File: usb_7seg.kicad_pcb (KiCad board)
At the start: 2 copper layers, 72 x 47 mm, 8 parts, among them IC1 MAX7219CNG, IC2 MAX7219CWG, U1 SeeeduinoXIAO, U2 7segment_led

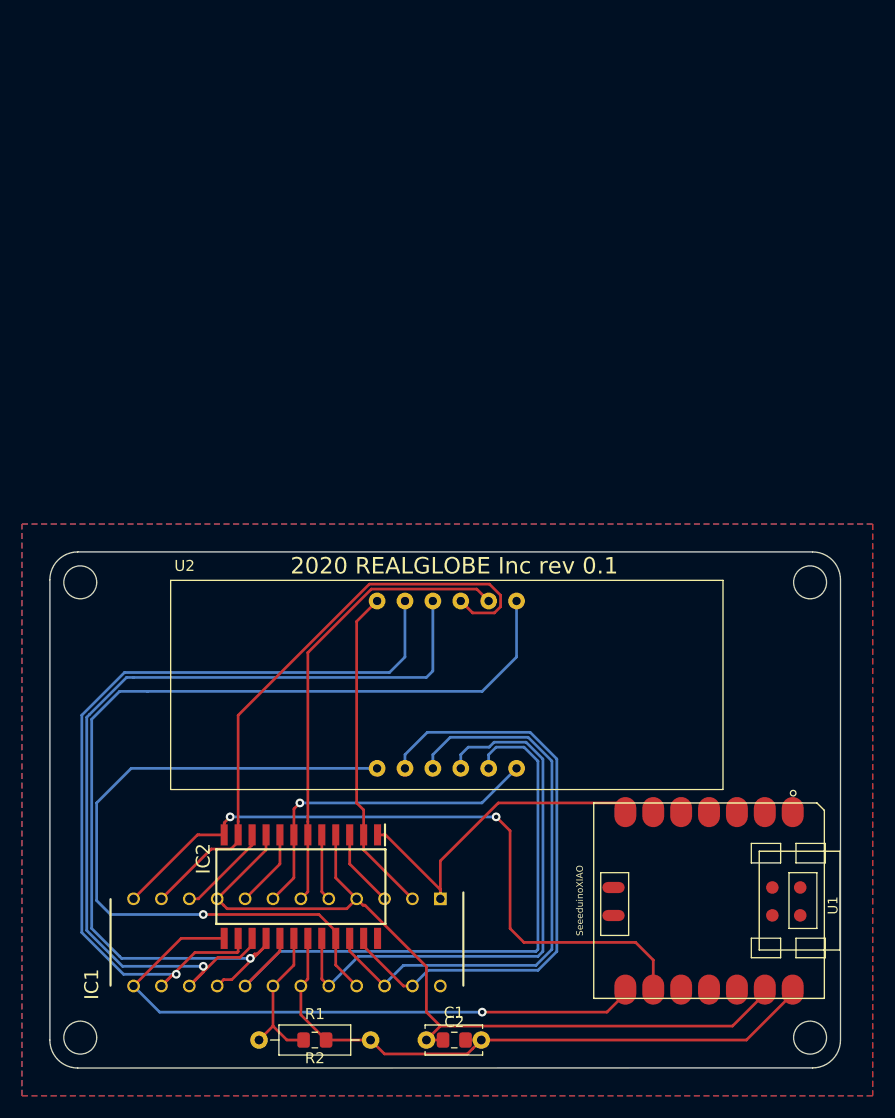
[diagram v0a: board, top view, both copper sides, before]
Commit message: いろいろ修正した
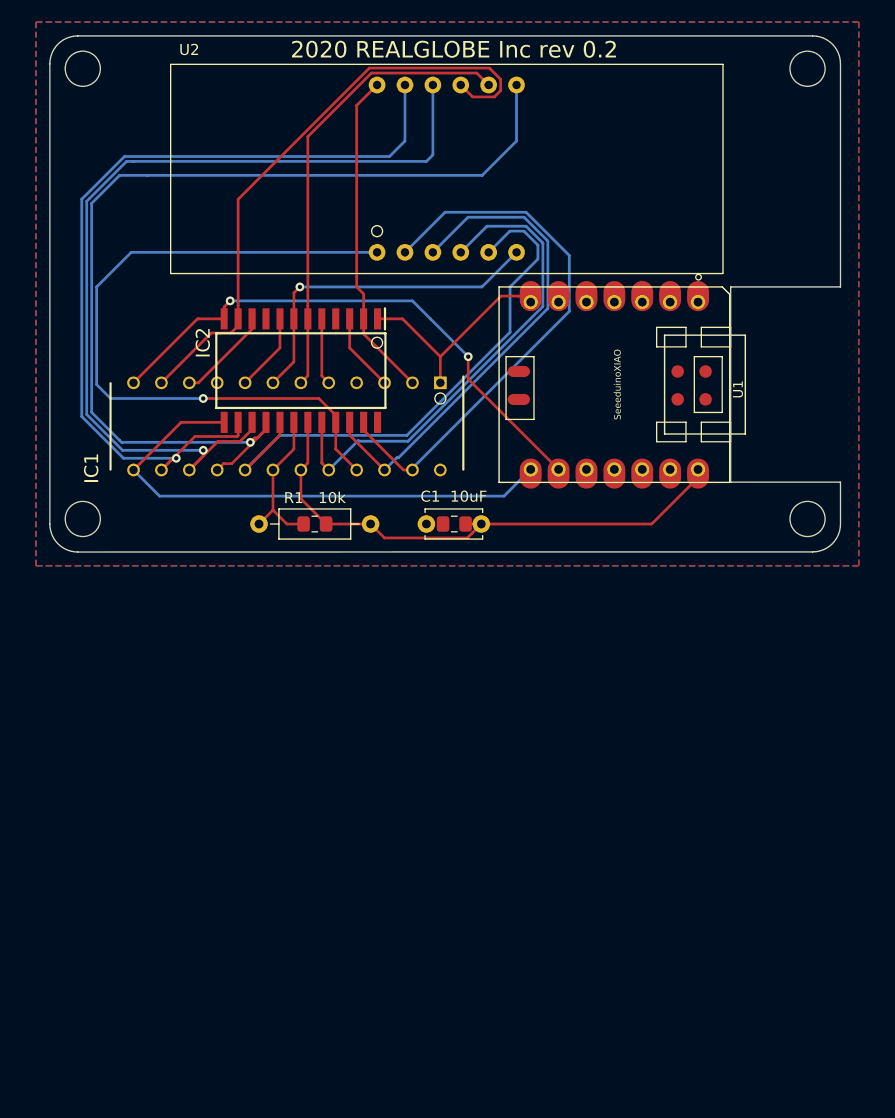
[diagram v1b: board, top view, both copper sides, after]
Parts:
- C1  10uF: renamed from C1
- R1   10k: renamed from R1
- U1: footprint Seeeduino XIAO:Seeeduino XIAO-MOUDLE14P-2.54-21X17.8MM -> kicad_mylib:SeeedXIAO
- U2: footprint kicad_7segment_led:kicad_7segment_led_0.56 -> kicad_mylib:7segment_led_0.56
- moved U1 47.8 mm to (40.9, -24.1)
- moved C1  10uF 47.0 mm to (34.3, -2.54)
- moved IC1 47.0 mm to (21.6, -11.4)
- moved IC2 47.0 mm to (22.9, -16.5)
- moved R1   10k 47.0 mm to (19.1, -2.54)
- moved ~ 47.0 mm to (36.8, -2.54)
- moved ~ 47.0 mm to (24.1, -2.54)
- moved U2 47.0 mm to (11.0, -25.4)
- renumbered C2 to ~, R2 to ~
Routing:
- net GND: track 77.0 -> 0.00 mm
- net Net-(IC1-Pad12): track 64.4 -> 50.0 mm
- net Net-(IC1-Pad1): track 32.0 -> 20.3 mm
- net Net-(IC1-Pad13): track 56.9 -> 48.2 mm, vias 1 -> 0
- net +5V: track 57.6 -> 49.0 mm
- net Net-(IC1-Pad17): track 57.4 -> 49.8 mm
- net Net-(IC1-Pad20): track 52.8 -> 45.3 mm
- net Net-(IC1-Pad22): track 53.8 -> 46.5 mm
- net Net-(IC1-Pad23): track 56.4 -> 50.9 mm
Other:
- outline, holes or cut-outs redrawn
- board text added: "2020 REALGLOBE Inc rev 0.2"
- board text removed: "2020 REALGLOBE Inc rev 0.1"
